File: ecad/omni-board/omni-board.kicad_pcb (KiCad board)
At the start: 2 copper layers, 6 parts, among them J1 Motor_BTS7960_01, J2 Motor_BTS7960_02, J3 Motor_BTS7960_03, J4 Motor_BTS7960_04, U1 ESP32-S3-Zero, U2 ESP32-S3-DevKitC

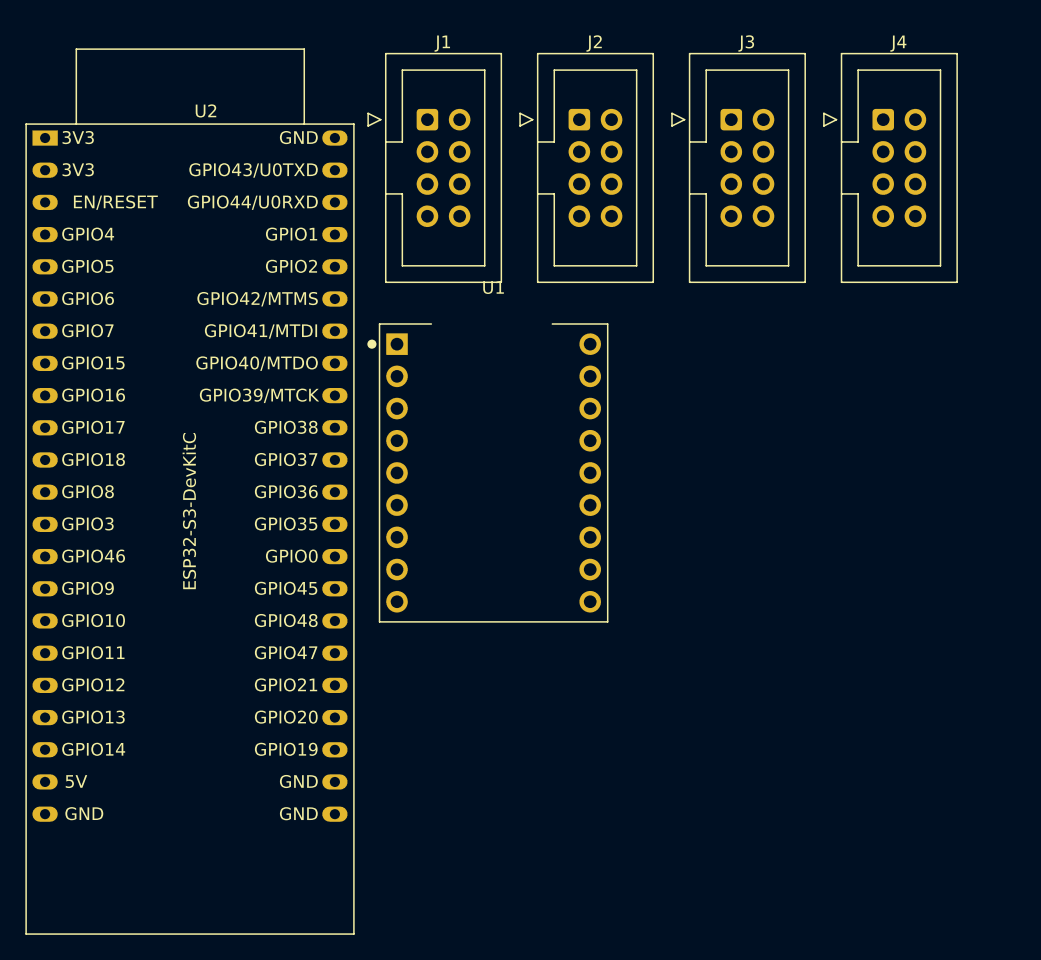
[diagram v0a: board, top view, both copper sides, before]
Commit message: update for production
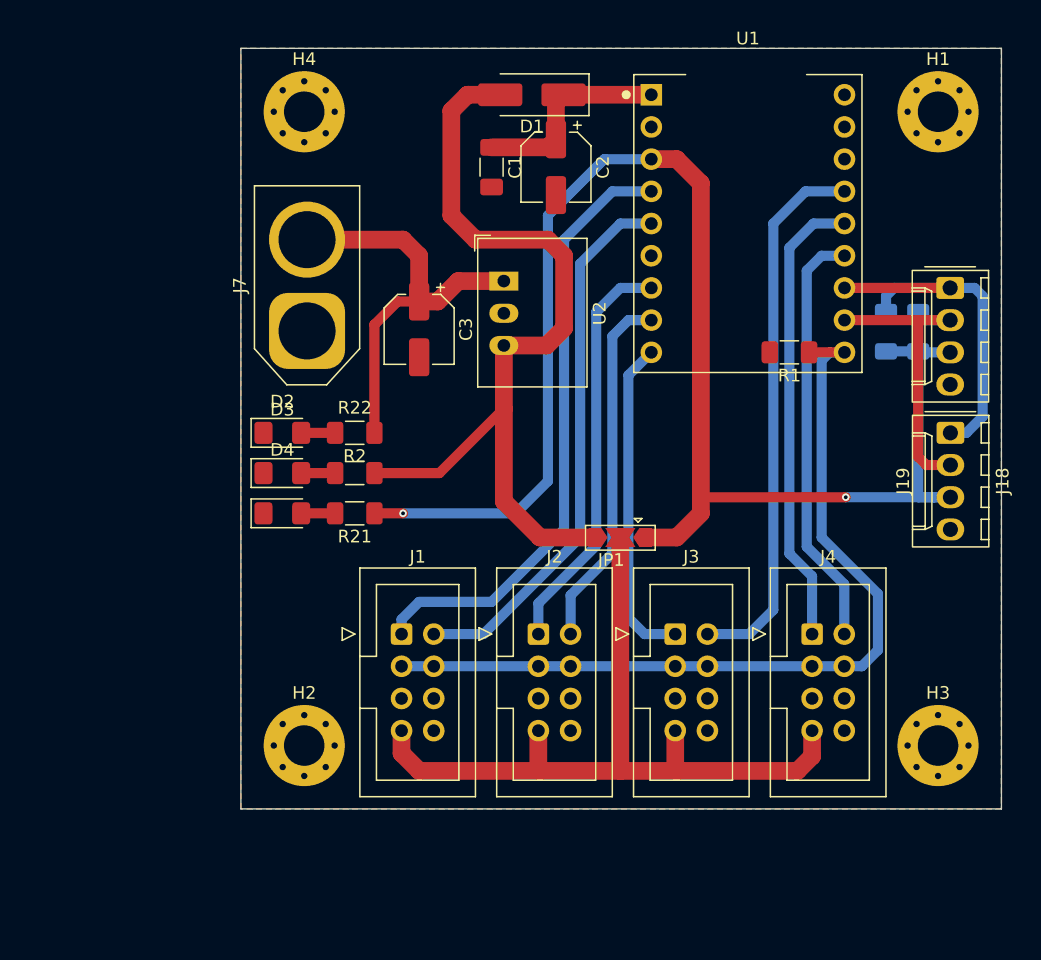
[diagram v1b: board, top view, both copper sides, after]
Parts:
- added C1: 0.1uF, Capacitor_SMD:C_1206_3216Metric_Pad1.33x1.80mm_HandSolder, F.Cu at (144.8, 79.4)
- added C2: 1uF, Capacitor_SMD:CP_Elec_5x5.4, F.Cu at (149.9, 79.4)
- added C3: 22uF, Capacitor_SMD:CP_Elec_5x5.4, F.Cu at (139.1, 92.2)
- added D1: SS14, Diode_SMD:D_SMA_Handsoldering, F.Cu at (148.0, 73.7)
- added D2: LED_Small, LED_SMD:LED_1206_3216Metric_Pad1.42x1.75mm_HandSolder, F.Cu at (128.3, 106.7)
- added D3: LED_Small, LED_SMD:LED_1206_3216Metric_Pad1.42x1.75mm_HandSolder, F.Cu at (128.3, 100.3)
- added D4: LED_Small, LED_SMD:LED_1206_3216Metric_Pad1.42x1.75mm_HandSolder, F.Cu at (128.3, 103.5)
- added H1: MountingHole_Pad, MountingHole:MountingHole_3.2mm_M3_Pad_Via, F.Cu at (180.0, 75.0)
- added H2: MountingHole_Pad, MountingHole:MountingHole_3.2mm_M3_Pad_Via, F.Cu at (130.0, 125.0)
- added H3: MountingHole_Pad, MountingHole:MountingHole_3.2mm_M3_Pad_Via, F.Cu at (180.0, 125.0)
- added H4: MountingHole_Pad, MountingHole:MountingHole_3.2mm_M3_Pad_Via, F.Cu at (130.0, 75.0)
- added J18: Conn_01x04, Connector_Molex:Molex_KK-254_AE-6410-04A_1x04_P2.54mm_Vertical, F.Cu at (181.0, 100.3)
- added J19: Conn_01x04, Connector_Molex:Molex_KK-254_AE-6410-04A_1x04_P2.54mm_Vertical, F.Cu at (181.0, 88.9)
- added J7: Con Batt, Connector_AMASS:AMASS_XT60-M_1x02_P7.20mm_Vertical, F.Cu at (130.2, 92.3)
- added JP1: SolderJumper_3_Open, Jumper:SolderJumper-3_P2.0mm_Open_TrianglePad1.0x1.5mm, F.Cu at (154.9, 108.6)
- added R1: 10k, Resistor_SMD:R_1206_3216Metric_Pad1.30x1.75mm_HandSolder, F.Cu at (168.3, 94.0)
- added R18: 10k, Resistor_SMD:R_1206_3216Metric_Pad1.30x1.75mm_HandSolder, B.Cu at (178.4, 92.4)
- added R19: 10k, Resistor_SMD:R_1206_3216Metric_Pad1.30x1.75mm_HandSolder, B.Cu at (175.9, 92.4)
- added R2: 1k, Resistor_SMD:R_1206_3216Metric_Pad1.30x1.75mm_HandSolder, F.Cu at (134.0, 100.3)
- added R21: 1k, Resistor_SMD:R_1206_3216Metric_Pad1.30x1.75mm_HandSolder, F.Cu at (134.0, 106.7)
- added R22: 1k, Resistor_SMD:R_1206_3216Metric_Pad1.30x1.75mm_HandSolder, F.Cu at (134.0, 103.5)
- U2: value ESP32-S3-DevKitC -> R-78E5.0-1.0; footprint PCM_Espressif:ESP32-S3-DevKitC -> Converter_DCDC:Converter_DCDC_RECOM_R-78E-0.5_THT
- moved J4 41.0 mm to (170.1, 116.2)
- moved J3 40.8 mm to (159.3, 116.2)
- moved J2 40.7 mm to (148.5, 116.2)
- moved J1 40.6 mm to (137.7, 116.2)
- moved U2 37.9 mm to (145.7, 88.4), turned to -90 degrees
- moved U1 28.1 mm to (165.0, 83.8)
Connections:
- U1 pad 1: unconnected-(U1-5V-Pad1) -> Net-(D1-K)
- U1 pad 10: L_PWM_03 -> EN_MOTORS
- U1 pad 13: R_PWM_04 -> L_PWM_04
- U1 pad 14: L_PWM_04 -> R_PWM_04
- U1 pad 15: EN_MOTORS -> L_PWM_03
- U2 pad 1: Net-(U2-3V3-Pad1) -> +12V
- U2 pad 2: Net-(U2-3V3-Pad1) -> GND
- U2 pad 3: unconnected-(U2-CHIP_PU-Pad3) -> +5V
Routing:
- net +3.3V: track 0.00 -> 120.4 mm, vias 0 -> 2
- net EN_MOTORS: track 0.00 -> 67.7 mm
- net +5V: track 0.00 -> 66.9 mm
- net VCC: track 0.00 -> 62.1 mm
- net R_PWM_01: track 0.00 -> 48.2 mm
- net L_PWM_01: track 0.00 -> 43.2 mm
- net L_PWM_03: track 0.00 -> 43.1 mm
- net R_PWM_04: track 0.00 -> 36.4 mm
- net L_PWM_04: track 0.00 -> 33.4 mm
- net +12V: track 0.00 -> 33.1 mm
- net R_PWM_02: track 0.00 -> 32.4 mm
- net SCL: track 0.00 -> 30.3 mm
- net L_PWM_02: track 0.00 -> 28.5 mm
- net R_PWM_03: track 0.00 -> 25.9 mm
- net SDA: track 0.00 -> 24.7 mm
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- added copper zone on B.Cu, net GND
- added copper zone on F.Cu, net GND
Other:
- board outline added: 60 x 60 mm
